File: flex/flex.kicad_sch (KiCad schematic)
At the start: 139 parts, among them J1 NA_Conn_01x06_Female, J2 NA_Conn_01x05_Female, J3 NA_Conn_01x06_Female, J4 NA_Conn_01x03_Female, J5 NA_Conn_01x03_Female, SW1 SW_Push, SW10 SW_Push, SW11 SW_Push, SW12 SW_Push, SW13 SW_Push, SW14 SW_Push, SW15 SW_Push, SW16 SW_Push, SW17 SW_Push, SW18 SW_Push, SW19 SW_Push, SW2 SW_Push, SW20 SW_Push, SW21 SW_Push, SW22 SW_Push, SW23 SW_Push, SW24 SW_Push, SW3 SW_Push, SW4 SW_Push, SW5 SW_Push, SW6 SW_Push, SW7 SW_Push, SW8 SW_Push, SW9 SW_Push

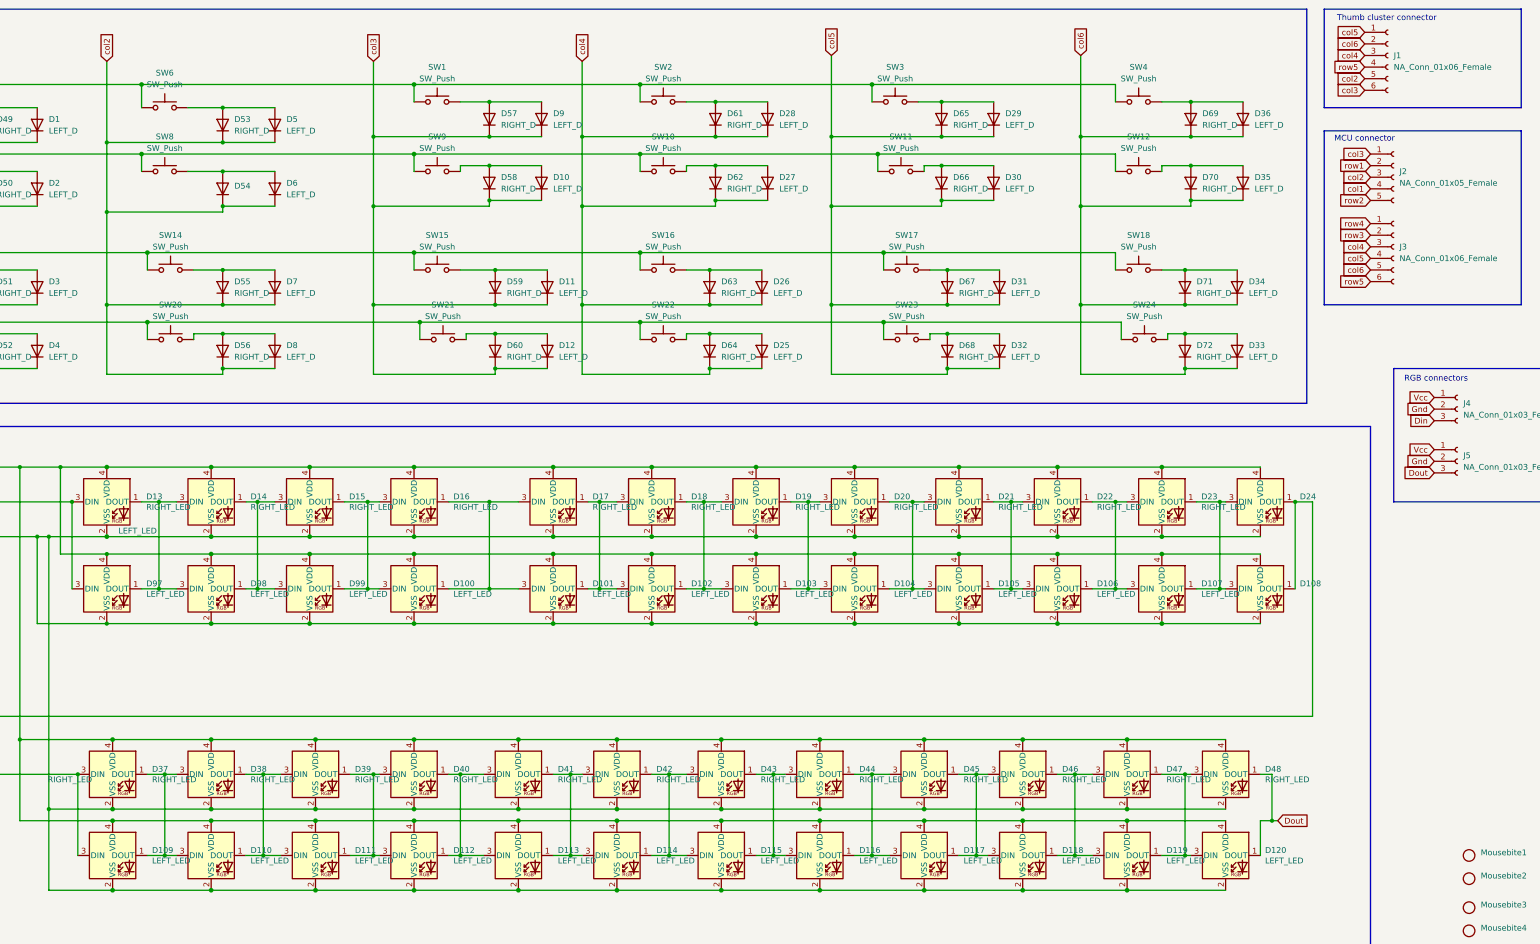
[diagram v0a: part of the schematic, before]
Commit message: BOM work
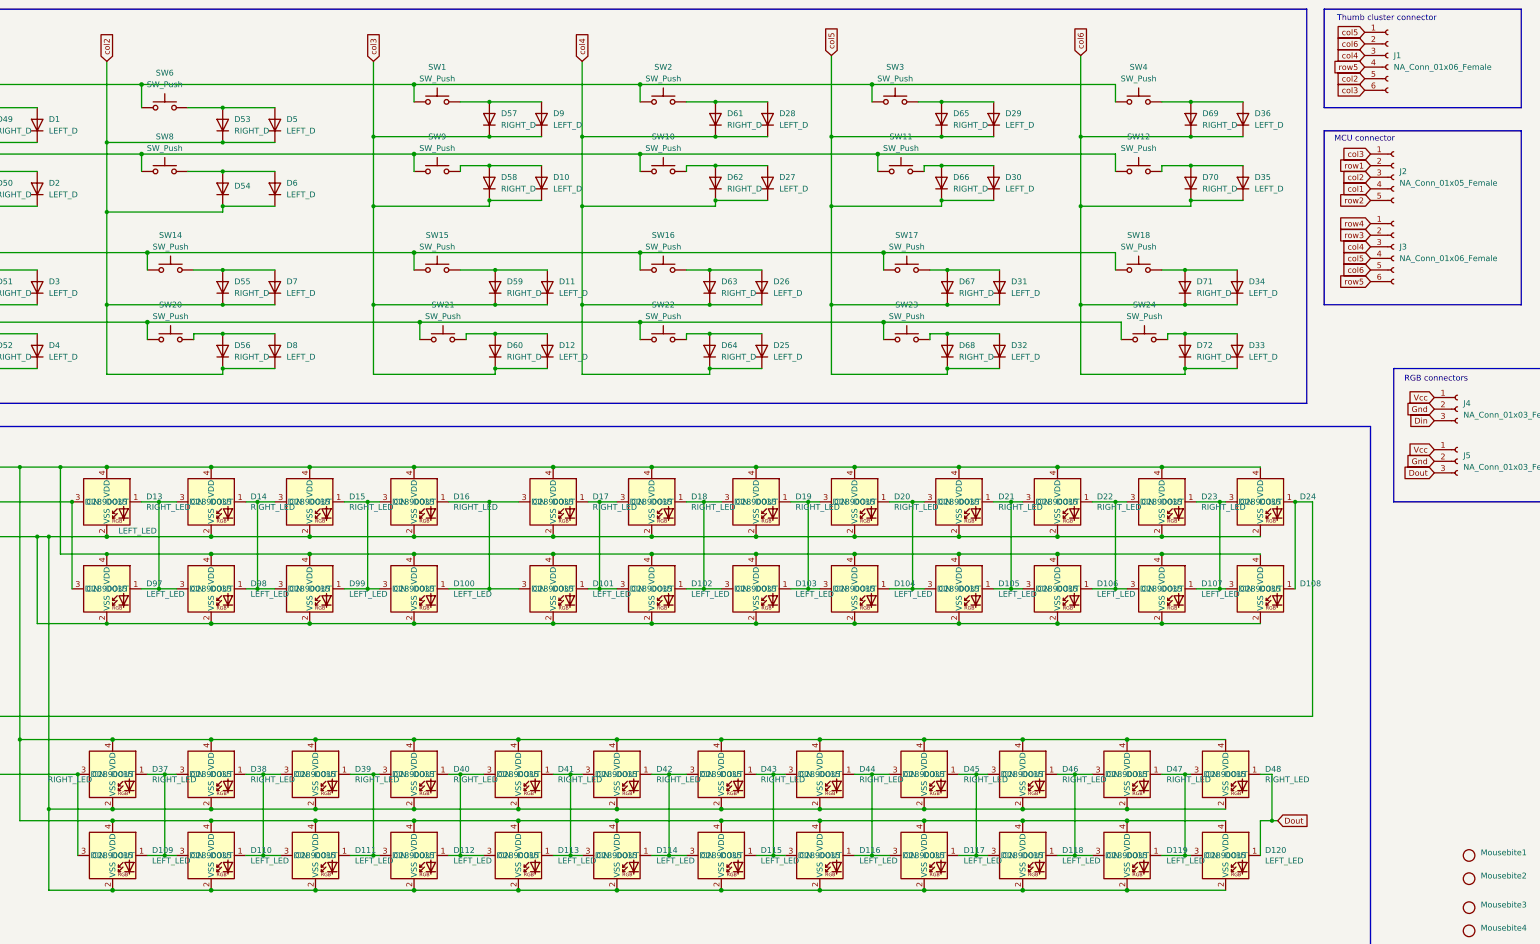
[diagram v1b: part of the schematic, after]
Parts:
- D1, D10, D11, D12, D2, D25, D26, D27, D28, D29, D3, D30, D31, D32, D33, D34, D35, D36, D4, D49, D5, D50, D51, D52, D53, D54, D55, D56, D57, D58, D59, D6, D60, D61, D62, D63, D64, D65, D66, D67, D68, D69, D7, D70, D71, D72, D8, D9: now in the parts list
- D100, D101, D102, D103, D104, D105, D106, D107, D108, D109, D110, D111, D112, D113, D114, D115, D116, D117, D118, D119, D120, D13, D14, D15, D16, D17, D18, D19, D20, D21, D22, D23, D24, D37, D38, D39, D40, D41, D42, D43, D44, D45, D46, D47, D48, D97, D98, D99: LCSC (none) -> C2890035
